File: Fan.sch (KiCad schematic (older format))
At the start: 9 parts

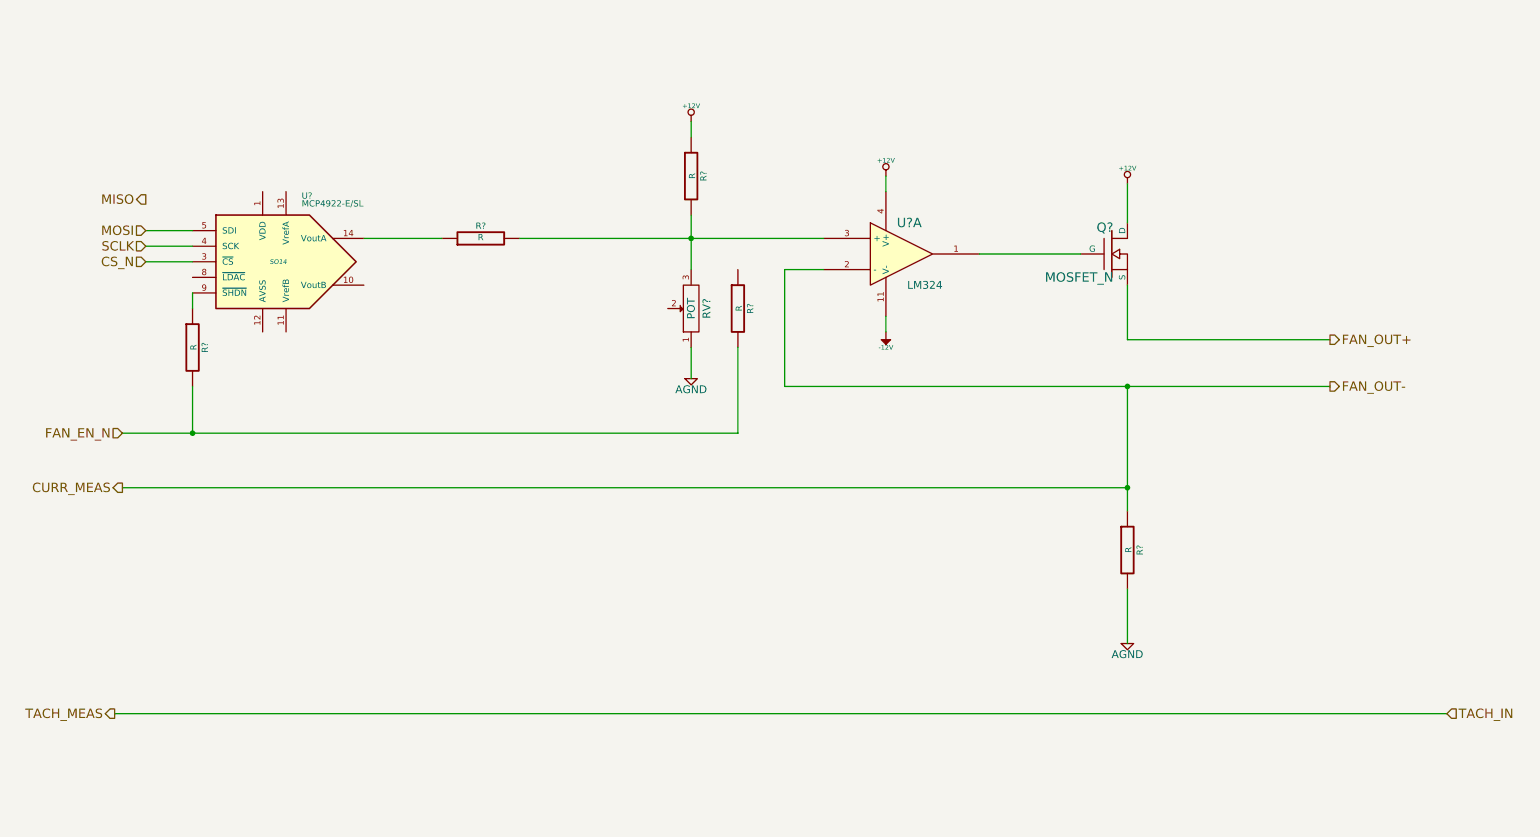
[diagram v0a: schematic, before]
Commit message: Revisting the Current/Fan Module
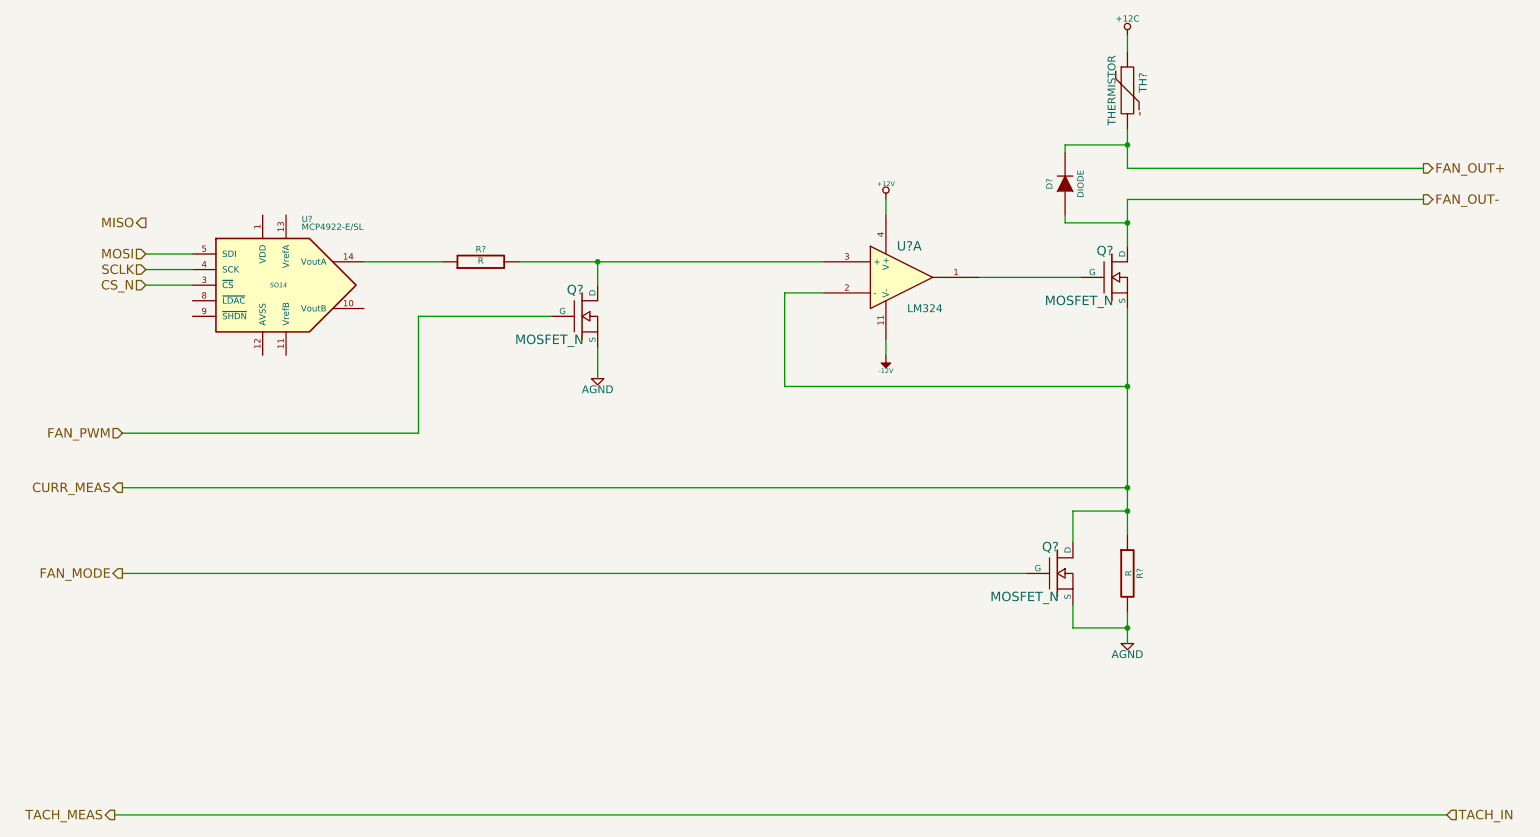
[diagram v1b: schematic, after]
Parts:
- removed R? (x3): R, symbol R
- removed RV?: POT, symbol POT
- added D?: DIODE, symbol DIODE
- added Q? (x2): MOSFET_N, symbol MOSFET_N
- added TH?: THERMISTOR, symbol THERMISTOR
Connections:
- net +12V: no longer Q?.D
- net AGND: now also Q?.S, Q?.S
- net CURR_MEAS: now also Q?.S, Q?.D
- net FAN_OUT+: now also D?.2 (K), TH?.2; no longer Q?.S
- net at R?.2, U?.3 (+): now also Q?.D
- new net +12C: TH?.1
- new net FAN_MODE: Q?.G
- new net FAN_OUT-: D?.1 (A), Q?.D
- new net FAN_PWM: Q?.G
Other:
- moved on the sheet: Q?, R?, U?, U?A
